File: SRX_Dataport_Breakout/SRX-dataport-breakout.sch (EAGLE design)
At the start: 15 parts

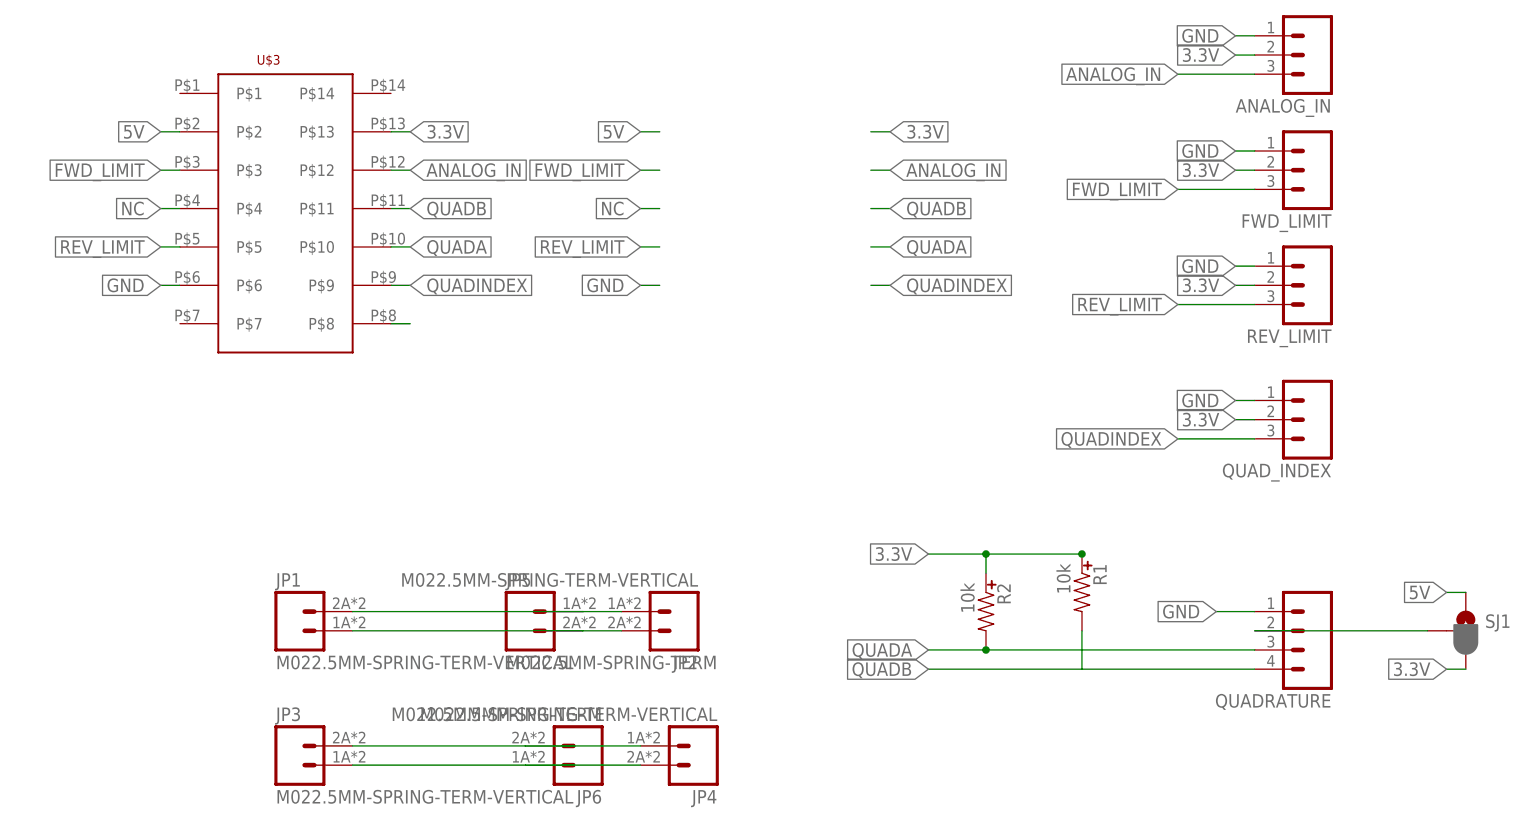
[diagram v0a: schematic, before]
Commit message: Add documentation
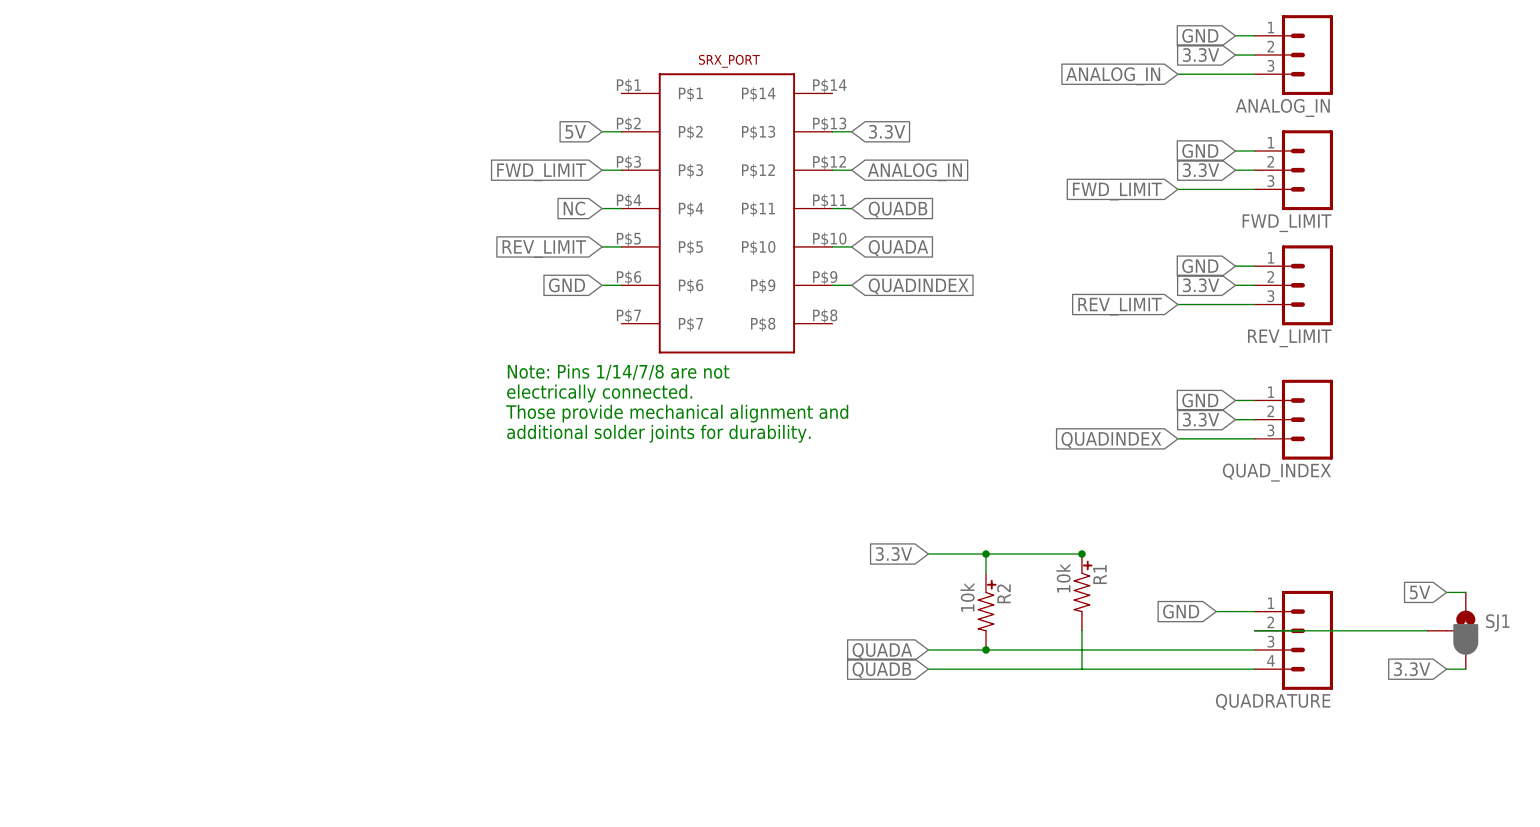
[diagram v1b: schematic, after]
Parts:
- removed JP1, JP2, JP3, JP4: M022.5MM-SPRING-TERM-VERTICAL, tekdemo:M022.5MM-SPRING-TERM-VERTICAL
- removed JP5, JP6: M022.5MM-SPRING-TERM, tekdemo:M022.5MM-SPRING-TERM
- removed U$3: M07X0220021321-00014TFLF, tekdemo:M07X0220021321-00014TFLF
- added SRX_PORT: M07X0220021321-00014TFLF, tekdemo:M07X0220021321-00014TFLF
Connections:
- removed net N$1: JP3.2, JP4.1, JP6.1
- removed net N$6: JP3.1, JP4.2, JP6.2
- removed net N$7: JP1.1, JP2.2, JP5.1
- removed net N$8: JP1.2, JP2.1, JP5.2
- net 3.3V: now also SRX_PORT.P$13; no longer U$3.P$13
- net 5V: now also SRX_PORT.P$2; no longer U$3.P$2
- net ANALOG_IN: now also SRX_PORT.P$12; no longer U$3.P$12
- net FWD_LIMIT: now also SRX_PORT.P$3; no longer U$3.P$3
- net GND: now also SRX_PORT.P$6; no longer U$3.P$6
- net NC: now also SRX_PORT.P$4; no longer U$3.P$4
- net QUADA: now also SRX_PORT.P$10; no longer U$3.P$10
- net QUADB: now also SRX_PORT.P$11; no longer U$3.P$11
- net QUADINDEX: now also SRX_PORT.P$9; no longer U$3.P$9
- net REV_LIMIT: now also SRX_PORT.P$5; no longer U$3.P$5
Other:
- note added: "Note: Pins 1/14/7/8 are not electrically connected. Those provide mechanical alignment and additional solder joints for durability."
